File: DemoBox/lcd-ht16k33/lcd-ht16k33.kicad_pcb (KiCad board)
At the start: 2 copper layers, 60 x 40 mm, 8 parts, among them J1 Conn_01x04, U1 HT16K33 24SOP, U2 3631AS, U3 3631AS

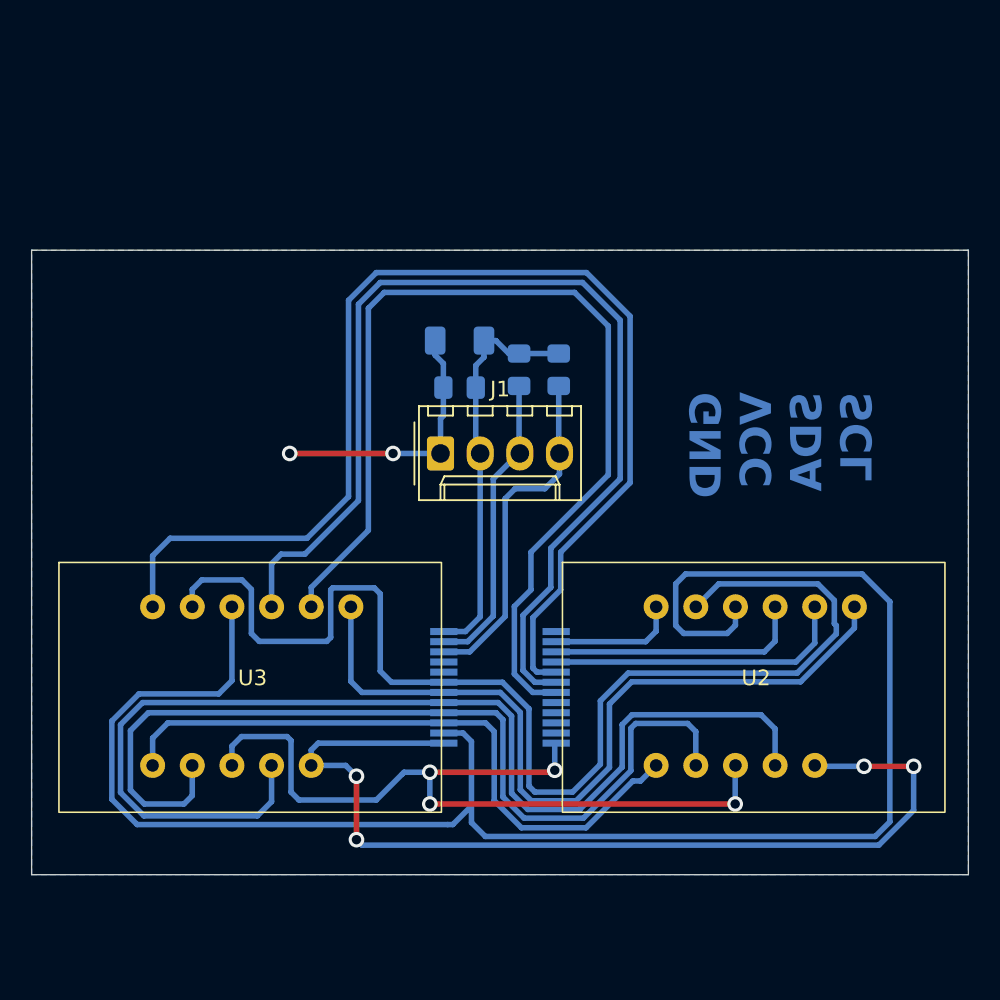
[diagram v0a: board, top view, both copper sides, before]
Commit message: refactor demobox
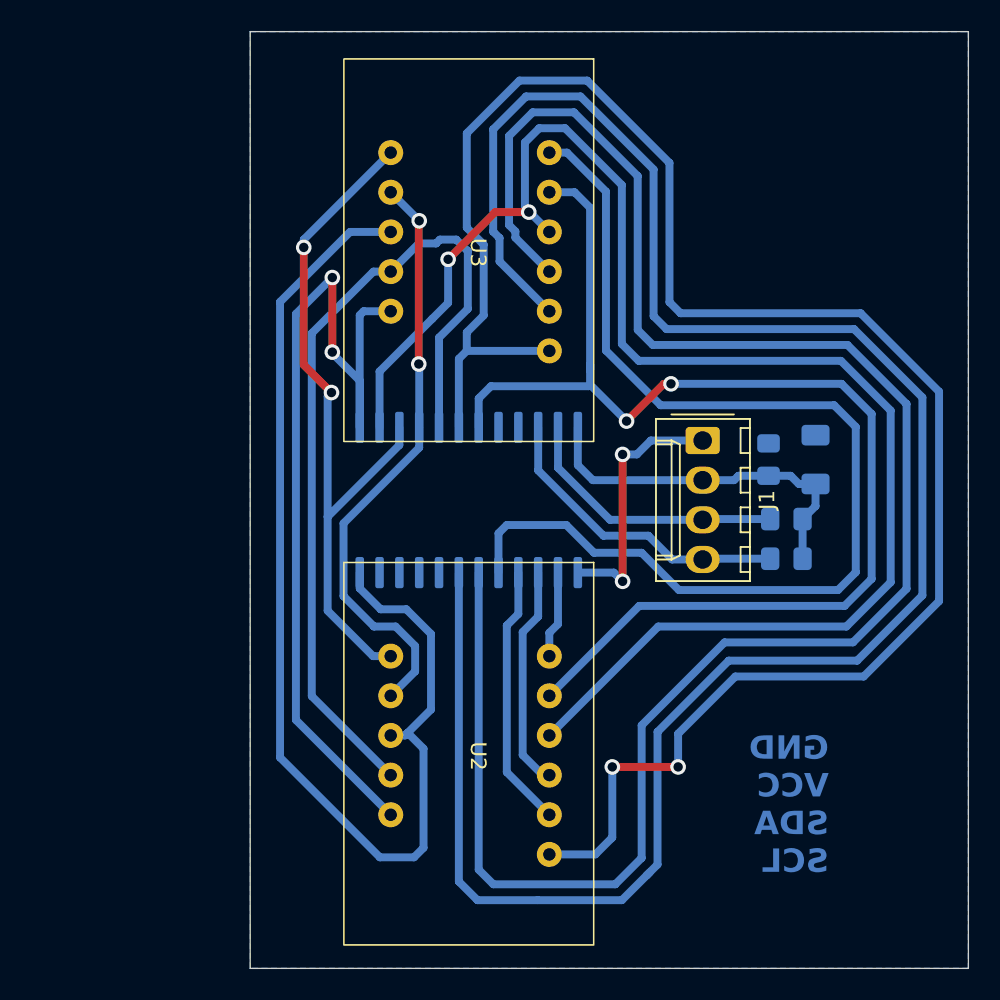
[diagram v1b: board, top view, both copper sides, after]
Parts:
- U1: footprint Package_SO:SSOP-24_5.3x8.2mm_P0.65mm -> Package_SO:SOP-24_7.5x15.4mm_P1.27mm
- moved U3 42.1 mm to (109.0, 35.8), turned to -90 degrees
- moved C1 24.0 mm to (136.2, 55.4), turned to 90 degrees
- moved C2 20.3 mm to (133.2, 55.4), turned to 90 degrees
- moved R1 19.6 mm to (134.3, 59.2), turned to 180 degrees
- moved R2 19.0 mm to (134.3, 61.8), turned to 180 degrees
- moved U2 18.4 mm to (109.0, 68.0), turned to -90 degrees
- moved J1 16.8 mm to (129.0, 54.2), turned to -90 degrees
- moved U1 12.2 mm to (114.0, 58.0), turned to 90 degrees
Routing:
- net /SEG2: track 51.4 -> 119.4 mm, vias 0 -> 2
- net /GR6: track 65.3 -> 131.0 mm
- net /GR5: track 68.4 -> 120.8 mm
- net /SEG4: track 59.2 -> 38.4 mm, vias 0 -> 2
- net /SEG8: track 52.4 -> 72.9 mm, vias 4 -> 0
- net /SEG3: track 72.4 -> 55.2 mm
- net /SEG6: track 114.4 -> 99.6 mm, vias 0 -> 2
- net /GR4: track 76.6 -> 70.0 mm
- net /SEG7: track 62.8 -> 57.5 mm, vias 4 -> 2
- net /SEG5: track 41.4 -> 45.4 mm, vias 0 -> 2
- net /COMMAND: track 8.24 -> 5.58 mm
- net /GR3: track 19.4 -> 16.9 mm
- net VCC: track 25.9 -> 23.5 mm
- net /SCL: track 22.2 -> 20.0 mm
- net /GR2: track 16.5 -> 14.3 mm
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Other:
- board size 60 x 40 mm -> 46 x 60 mm
